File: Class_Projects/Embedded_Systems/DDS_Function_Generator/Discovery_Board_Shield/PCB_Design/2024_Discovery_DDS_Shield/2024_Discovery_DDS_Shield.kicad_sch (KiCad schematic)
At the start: 66 parts, among them J1 FILTER_CONN, J2 10118194-0001LF, J3 FTDI_UART_CONN, J4 DC_OFFSET_CONN, J5 LCD_CONN, J6 Conn_OpAmp_Power, J7 Conn_DiscBoard_Right, J8 Conn_DiscBoard_Left, J9 BNC_CONN, SW2 SW_MODE, SW3 SW_CURSOR, SW4 SW_PLUS, SW5 SW_MINUS, SW6 SW_RUN_STOP, U1 TL072, U2 TL072, U5 FT230XS

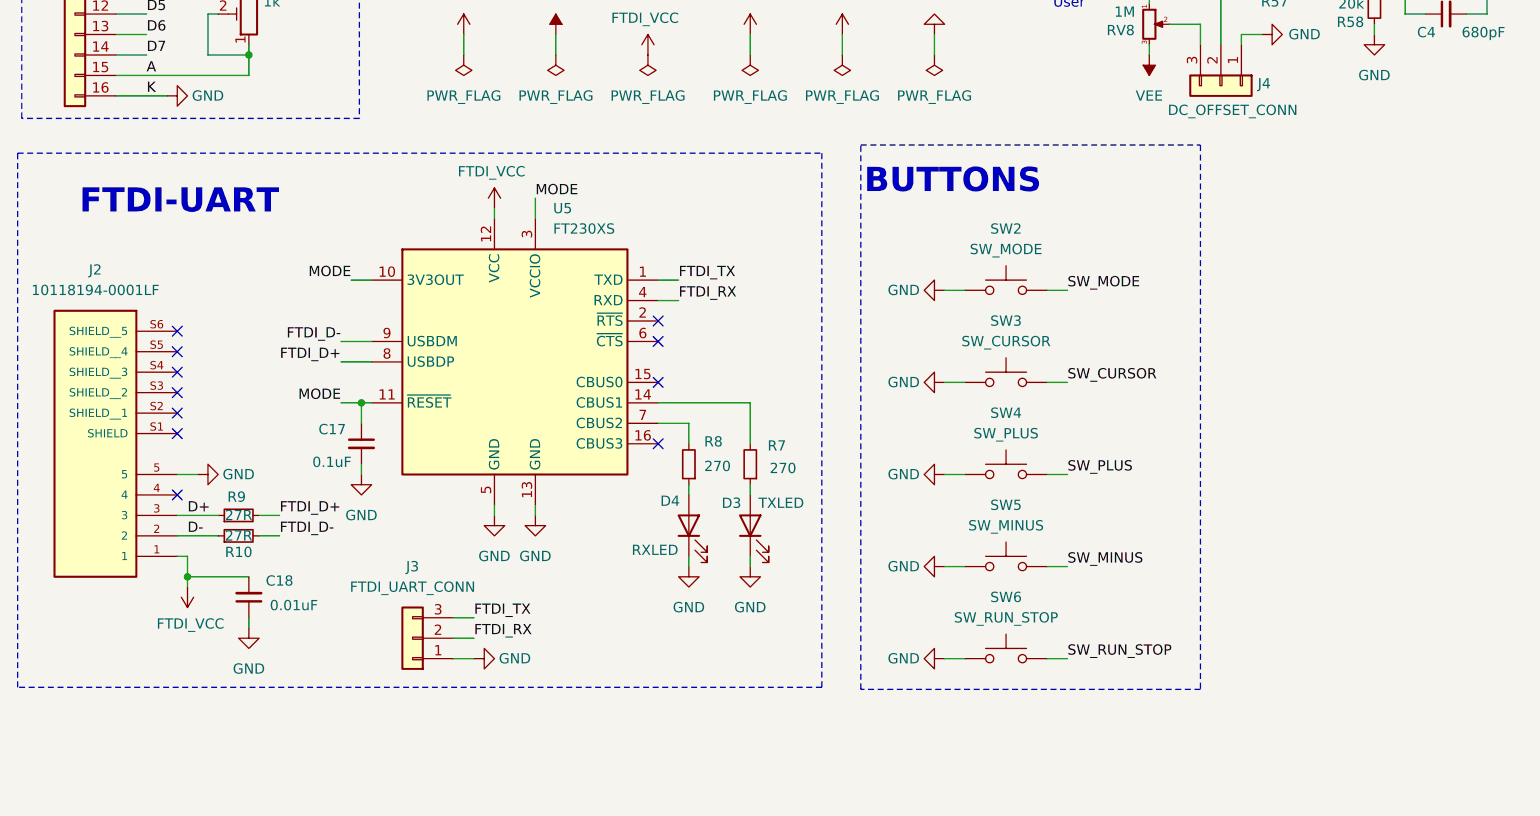
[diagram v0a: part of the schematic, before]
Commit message: new board version
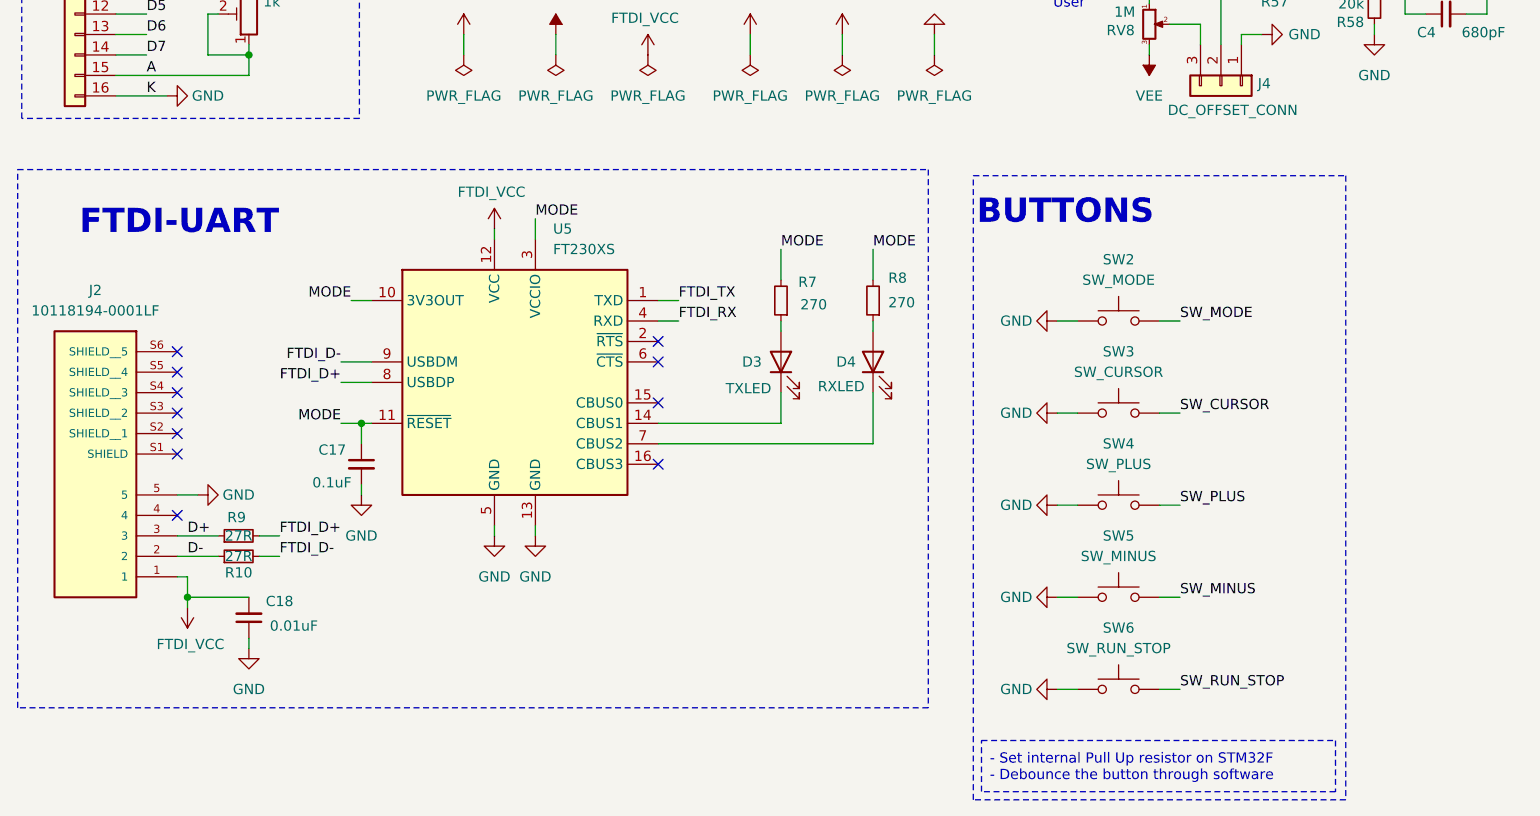
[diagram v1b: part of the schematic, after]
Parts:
- removed J3: FTDI_UART_CONN, Connector_PinHeader_2.54mm:PinHeader_1x03_P2.54mm_Vertical, symbol Connector_Generic:Conn_01x03
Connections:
- net GND: no longer D3.1 (K), D4.1 (K)
- net MODE: now also R7.2, R8.2
- net at U5.14 (CBUS1): now also D3.1 (K); no longer R7.2
- net at U5.7 (CBUS2): now also D4.1 (K); no longer R8.2
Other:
- moved on the sheet: C17, C18, D3, D4, J2, R10, R7, R8, R9, SW2, SW3, SW4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
